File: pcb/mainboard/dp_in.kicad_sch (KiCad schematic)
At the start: 32 parts, among them J601 USB_C_Receptacle, U601 PTN3460, U602 TPS2001D, U603 USBLC6-2P6, U604 FUSB302BMPX, U605 CBTL02043A

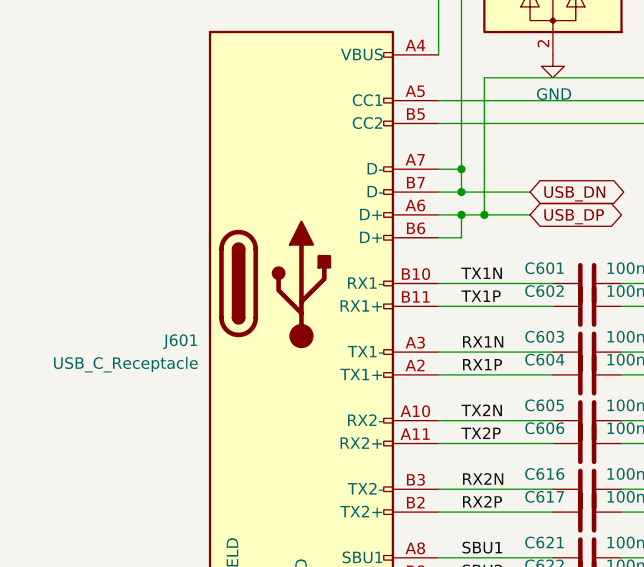
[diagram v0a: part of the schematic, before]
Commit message: pcb: r0p6
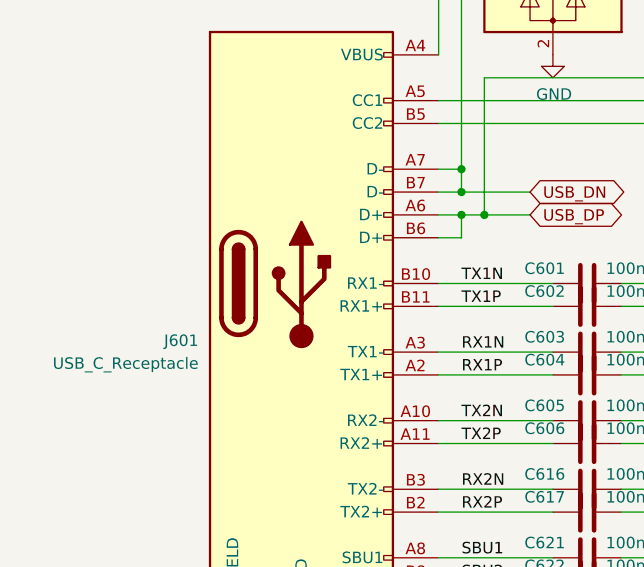
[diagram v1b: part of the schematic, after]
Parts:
- J601: footprint Connector_USB:USB_C_Receptacle_Amphenol_12401548E4-2A -> footprints:USB-306A-B-SU

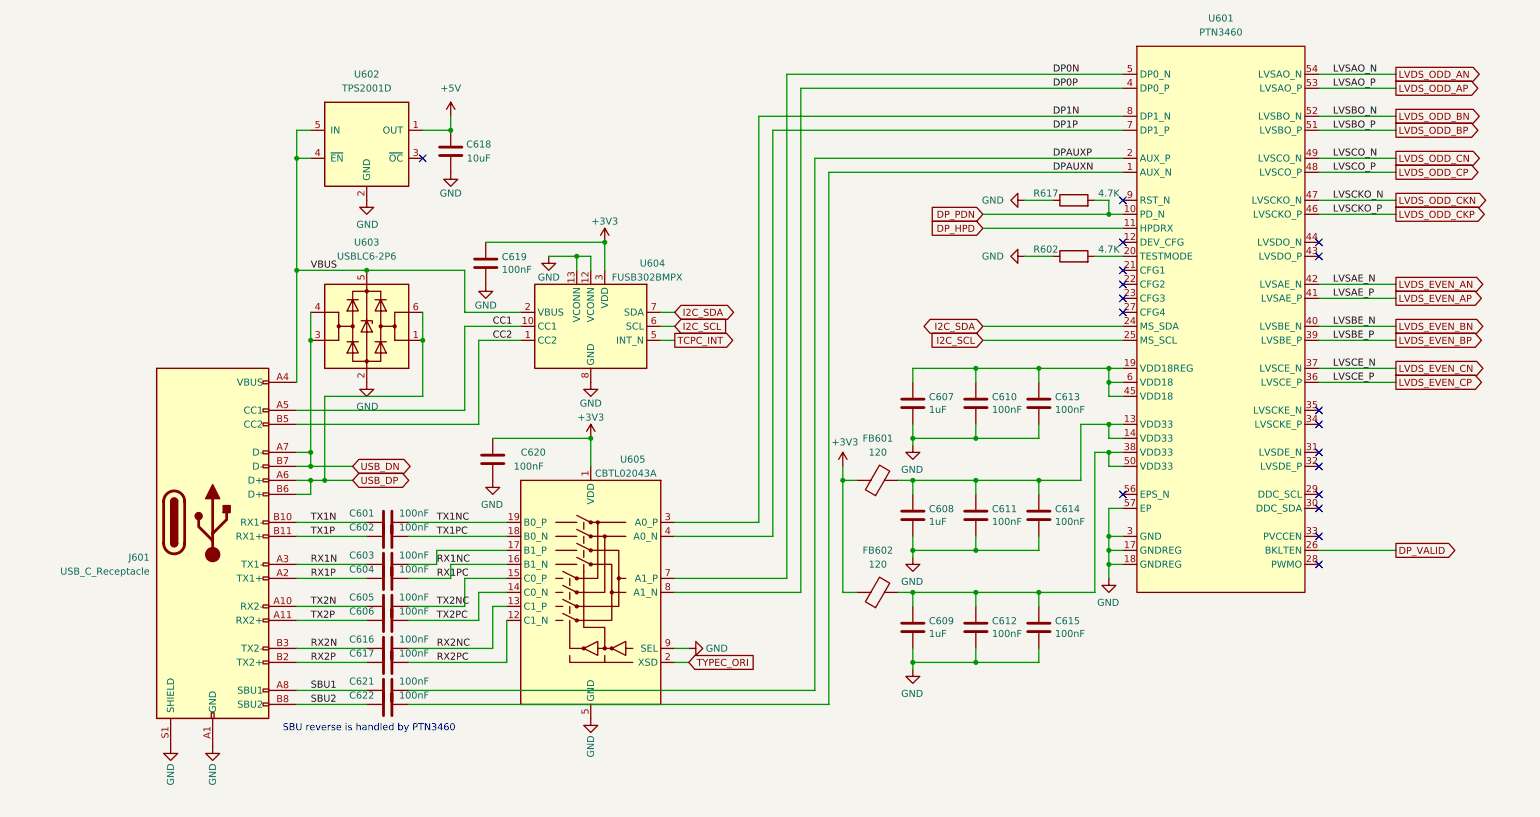
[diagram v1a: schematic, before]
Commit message: r0p7 wip, check in before switch to kicad 8
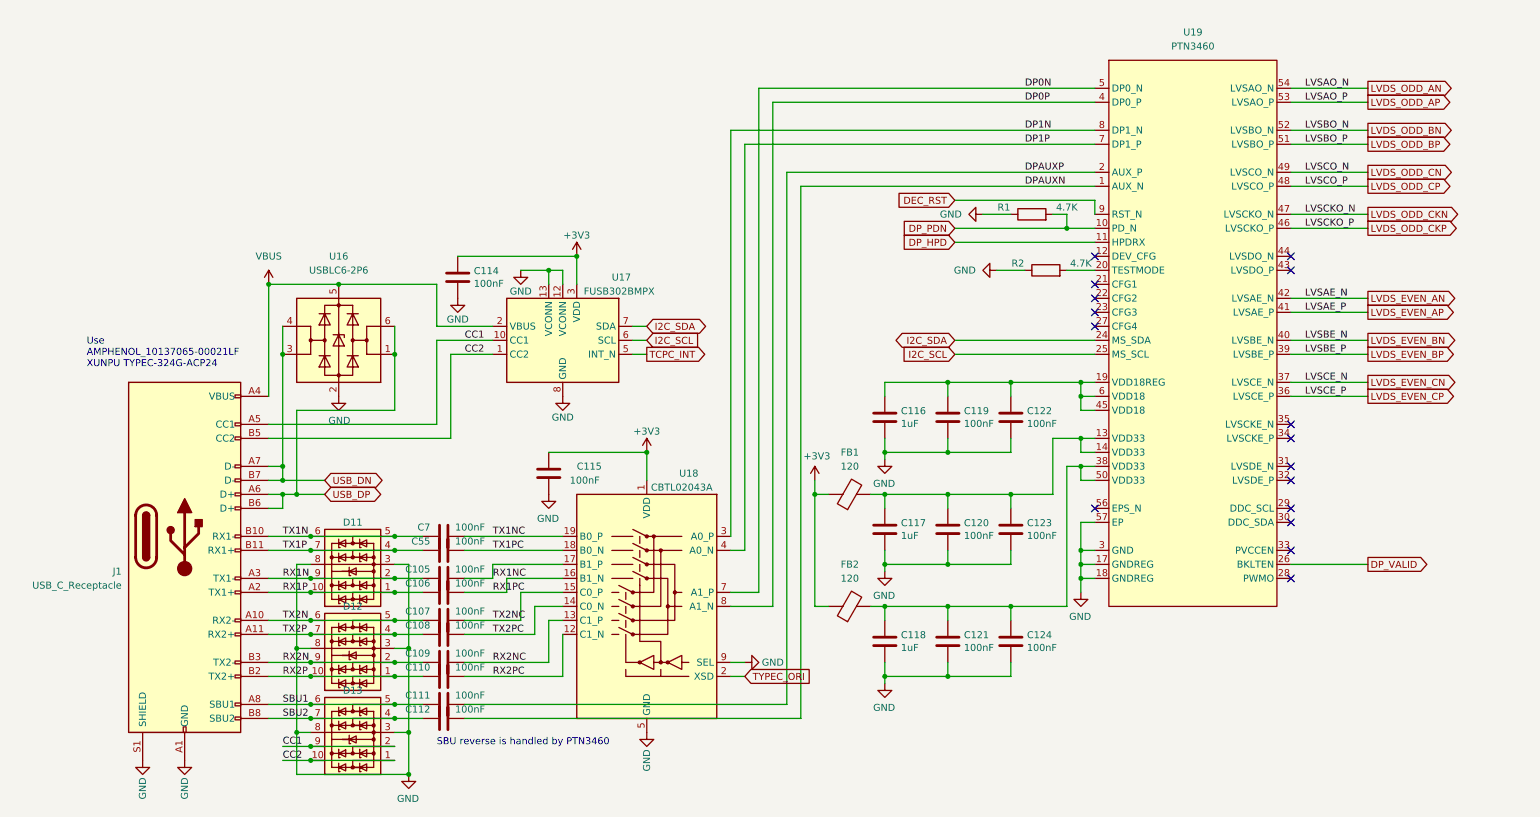
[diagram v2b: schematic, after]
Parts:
- removed C601, C602, C603, C604, C605, C606, C610, C611, C612, C613, C614, C615, C616, C617, C619, C620, C621, C622: 100nF, Capacitor_SMD:C_0402_1005Metric, symbol Device:C
- removed C607, C608, C609: 1uF, Capacitor_SMD:C_0402_1005Metric, symbol Device:C
- removed C618: 10uF, Capacitor_SMD:C_0603_1608Metric, symbol Device:C
- removed FB601, FB602: 120, Inductor_SMD:L_0603_1608Metric, symbol Device:FerriteBead
- removed J601: USB_C_Receptacle, footprints:USB-306A-B-SU, symbol Connector:USB_C_Receptacle
- removed R602, R617: 4.7K, Resistor_SMD:R_0402_1005Metric, symbol Device:R
- removed U601: PTN3460, Package_DFN_QFN:QFN-56-1EP_7x7mm_P0.4mm_EP5.6x5.6mm, symbol symbols:PTN3460
- removed U602: TPS2001D, Package_TO_SOT_SMD:SOT-23-5, symbol symbols:TPS2001D
- removed U603: USBLC6-2P6, Package_TO_SOT_SMD:SOT-666, symbol Power_Protection:USBLC6-2P6
- removed U604: FUSB302BMPX, Package_DFN_QFN:WQFN-14-1EP_2.5x2.5mm_P0.5mm_EP1.45x1.45mm, symbol Interface_USB:FUSB302BMPX
- removed U605: CBTL02043A, Package_DFN_QFN:WQFN-20-1EP_2.5x4.5mm_P0.5mm_EP1x2.9mm, symbol Analog_Switch:CBTL02043A
- added C105, C106, C107, C108, C109, C110, C111, C112, C114, C115, C119, C120, C121, C122, C123, C124, C55, C7: 100nF, Capacitor_SMD:C_0402_1005Metric, symbol Device:C
- added C116, C117, C118: 1uF, Capacitor_SMD:C_0402_1005Metric, symbol Device:C
- added D11, D12, D13: RCLAMP0524P, Package_DFN_QFN:Diodes_UDFN-10_1.0x2.5mm_P0.5mm, symbol symbols:RCLAMP0524P
- added FB1, FB2: 120, Inductor_SMD:L_0603_1608Metric, symbol Device:FerriteBead
- added J1: USB_C_Receptacle, footprints:AMPHENOL_10137065-00021LF, symbol Connector:USB_C_Receptacle
- added R1, R2: 4.7K, Resistor_SMD:R_0402_1005Metric, symbol Device:R
- added U16: USBLC6-2P6, Package_TO_SOT_SMD:SOT-666, symbol Power_Protection:USBLC6-2P6
- added U17: FUSB302BMPX, Package_DFN_QFN:WQFN-14-1EP_2.5x2.5mm_P0.5mm_EP1.45x1.45mm, symbol Interface_USB:FUSB302BMPX
- added U18: CBTL02043A, Package_DFN_QFN:WQFN-20-1EP_2.5x4.5mm_P0.5mm_EP1x2.9mm, symbol Analog_Switch:CBTL02043A
- added U19: PTN3460, Package_DFN_QFN:QFN-56-1EP_7x7mm_P0.4mm_EP5.6x5.6mm, symbol symbols:PTN3460
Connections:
- net +3V3: now also C114.1, C115.1, FB1.1, FB2.1, U17.3 (VDD), U17.4 (VDD), U18.1 (VDD), U18.10 (VDD), U18.6 (VDD)
- net CC1: now also D13.2 (IO2), D13.9 (NC3), J1.A5 (CC1), U17.10 (CC1), U17.11 (CC1)
- net CC2: now also D13.1 (IO1), D13.10 (NC4), J1.B5 (CC2), U17.1 (CC2), U17.14 (CC2)
- net DP0N: now also U18.7 (A1_P), U19.5 (DP0_N)
- net DP0P: now also U18.8 (A1_N), U19.4 (DP0_P)
- net DP1N: now also U18.3 (A0_P), U19.8 (DP1_N)
- net DP1P: now also U18.4 (A0_N), U19.7 (DP1_P)
- net DPAUXN: now also C112.2, U19.1 (AUX_N)
- net DPAUXP: now also C111.2, U19.2 (AUX_P)
- net DP_HPD: now also U19.11 (HPDRX)
- net DP_PDN: now also R1.2, U19.10 (PD_N)
- net DP_VALID: now also U19.26 (BKLTEN)
- net GND: now also C114.2, C115.2, C116.2, C117.2, C118.2, C119.2, C120.2, C121.2, C122.2, C123.2, C124.2, D11.3 (GND), D11.8 (GND), D12.3 (GND), D12.8 (GND), D13.3 (GND), D13.8 (GND), J1.A1 (GND), J1.A12 (GND), J1.B1 (GND), J1.B12 (GND), J1.S1 (SHIELD), R1.1, R2.1, U16.2 (GND), U17.12 (VCONN), U17.13 (VCONN), U17.15 (GND), U17.8 (GND), U17.9 (GND), U18.11 (GND), U18.20 (GND), U18.21 (GND), U18.5 (GND), U18.9 (SEL), U19.17 (GNDREG), U19.18 (GNDREG), U19.3 (GND), U19.57 (EP)
- net I2C_SCL: now also U17.6 (SCL), U19.25 (MS_SCL)
- net I2C_SDA: now also U17.7 (SDA), U19.24 (MS_SDA)
- net LVDS_EVEN_AN: now also U19.42 (LVSAE_N)
- net LVDS_EVEN_AP: now also U19.41 (LVSAE_P)
- net LVDS_EVEN_BN: now also U19.40 (LVSBE_N)
- net LVDS_EVEN_BP: now also U19.39 (LVSBE_P)
- net LVDS_EVEN_CN: now also U19.37 (LVSCE_N)
- net LVDS_EVEN_CP: now also U19.36 (LVSCE_P)
- net LVDS_ODD_AN: now also U19.54 (LVSAO_N)
- net LVDS_ODD_AP: now also U19.53 (LVSAO_P)
- net LVDS_ODD_BN: now also U19.52 (LVSBO_N)
- net LVDS_ODD_BP: now also U19.51 (LVSBO_P)
- net LVDS_ODD_CKN: now also U19.47 (LVSCKO_N)
- net LVDS_ODD_CKP: now also U19.46 (LVSCKO_P)
- net LVDS_ODD_CN: now also U19.49 (LVSCO_N)
- net LVDS_ODD_CP: now also U19.48 (LVSCO_P)
- net RX1N: now also C105.1, D11.2 (IO2), D11.9 (NC3), J1.A3 (TX1-)
- net RX1NC: now also C105.2, U18.17 (B1_P)
- net RX1P: now also C106.1, D11.1 (IO1), D11.10 (NC4), J1.A2 (TX1+)
- net RX1PC: now also C106.2, U18.16 (B1_N)
- net RX2N: now also C109.1, D12.2 (IO2), D12.9 (NC3), J1.B3 (TX2-)
- net RX2NC: now also C109.2, U18.13 (C1_P)
- net RX2P: now also C110.1, D12.1 (IO1), D12.10 (NC4), J1.B2 (TX2+)
- net RX2PC: now also C110.2, U18.12 (C1_N)
- net SBU1: now also C111.1, D13.5 (IO4), D13.6 (NC1), J1.A8 (SBU1)
- net SBU2: now also C112.1, D13.4 (IO3), D13.7 (NC2), J1.B8 (SBU2)
- net TCPC_INT: now also U17.5 (INT_N)
- net TX1N: now also C7.1, D11.5 (IO4), D11.6 (NC1), J1.B10 (RX1-)
- net TX1NC: now also C7.2, U18.19 (B0_P)
- net TX1P: now also C55.1, D11.4 (IO3), D11.7 (NC2), J1.B11 (RX1+)
- net TX1PC: now also C55.2, U18.18 (B0_N)
- net TX2N: now also C107.1, D12.5 (IO4), D12.6 (NC1), J1.A10 (RX2-)
- net TX2NC: now also C107.2, U18.15 (C0_P)
- net TX2P: now also C108.1, D12.4 (IO3), D12.7 (NC2), J1.A11 (RX2+)
- net TX2PC: now also C108.2, U18.14 (C0_N)
- net TYPEC_ORI: now also U18.2 (XSD)
- net USB_DN: now also J1.A7 (D-), J1.B7 (D-), U16.3 (I/O2), U16.4 (I/O2)
- net USB_DP: now also J1.A6 (D+), J1.B6 (D+), U16.1 (I/O1), U16.6 (I/O1)
- net VBUS: now also J1.A4 (VBUS), J1.A9 (VBUS), J1.B4 (VBUS), J1.B9 (VBUS), U16.5 (VBUS), U17.2 (VBUS)
- new net: C116.1, C119.1, C122.1, U19.19 (VDD18REG), U19.45 (VDD18), U19.6 (VDD18)
- new net: C118.1, C121.1, C124.1, FB2.2, U19.38 (VDD33), U19.50 (VDD33)
- new net: C117.1, C120.1, C123.1, FB1.2, U19.13 (VDD33), U19.14 (VDD33)
- new net: R2.2, U19.20 (TESTMODE)
- new net DEC_RST: U19.9 (RST_N)
- no-connect marks 18 -> 16
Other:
- note added: "Use AMPHENOL_10137065-00021LF XUNPU TYPEC-324G-ACP24"

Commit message: r0p7 wip
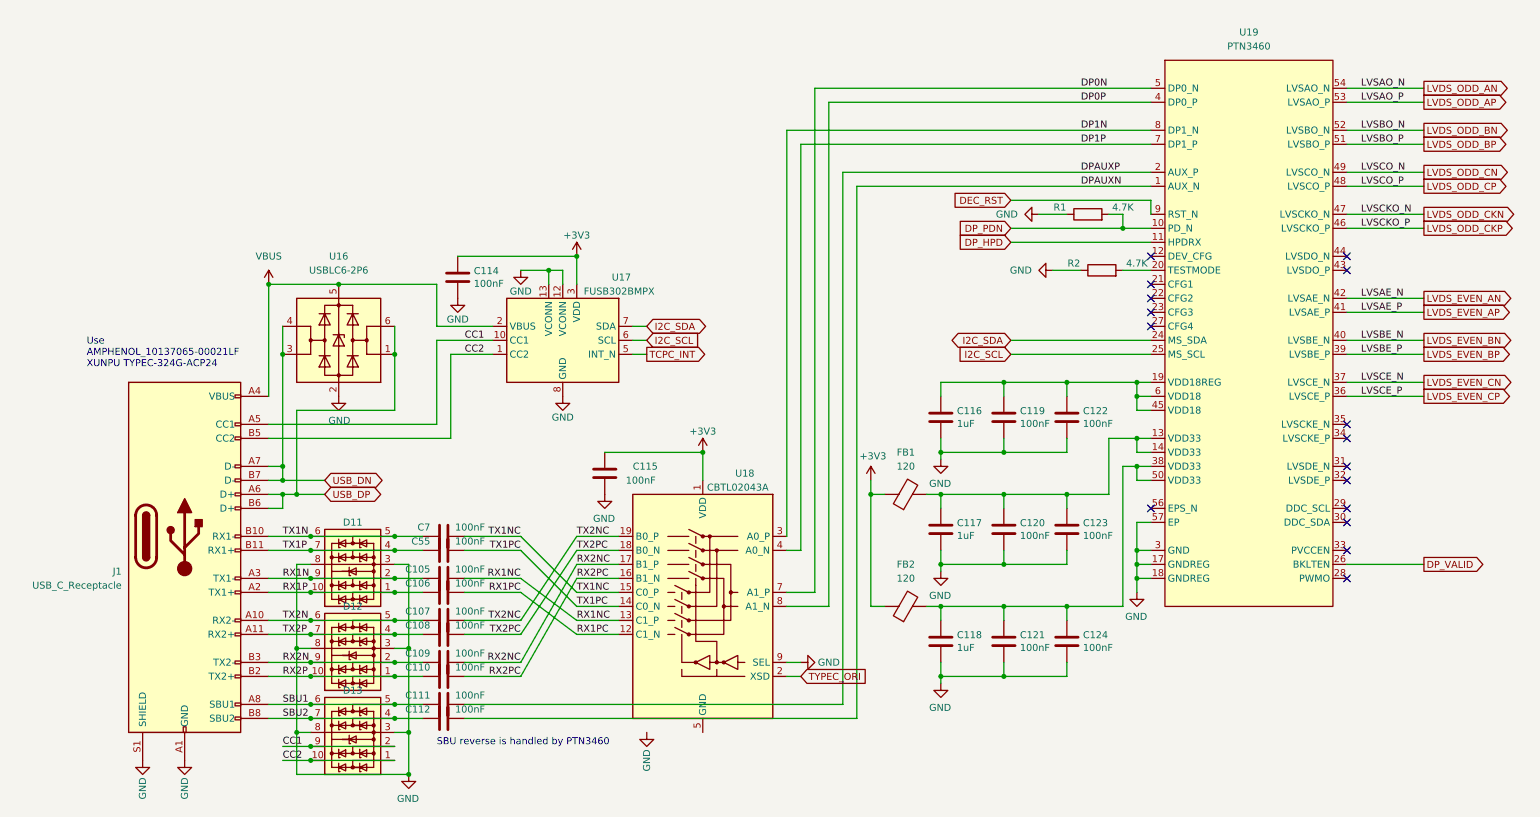
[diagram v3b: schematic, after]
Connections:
- net GND: no longer U18.11 (GND), U18.20 (GND), U18.21 (GND), U18.5 (GND)
- net RX1NC: now also U18.13 (C1_P); no longer U18.17 (B1_P)
- net RX1PC: now also U18.12 (C1_N); no longer U18.16 (B1_N)
- net RX2NC: now also U18.17 (B1_P); no longer U18.13 (C1_P)
- net RX2PC: now also U18.16 (B1_N); no longer U18.12 (C1_N)
- net TX1NC: now also U18.15 (C0_P); no longer U18.19 (B0_P)
- net TX1PC: now also U18.14 (C0_N); no longer U18.18 (B0_N)
- net TX2NC: now also U18.19 (B0_P); no longer U18.15 (C0_P)
- net TX2PC: now also U18.18 (B0_N); no longer U18.14 (C0_N)
- new net: U18.11 (GND), U18.20 (GND), U18.21 (GND), U18.5 (GND)
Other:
- moved on the sheet: C115, C116, C117, C118, C119, C120, C121, C122, C123, C124, FB1, FB2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
